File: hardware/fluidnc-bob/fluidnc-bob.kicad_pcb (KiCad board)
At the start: 2 copper layers, 45 parts, among them J1 5V-IN, J10 LIM-Z, J11 PROBE, J2 X-DRV, J3 Y-DRV, J4 Z-DRV, J5 LIM-X, J6 LIM-Y, J7 RELAY, J8 AUX, J9 SD, Q1 2N7000, U1 SN74HC541N

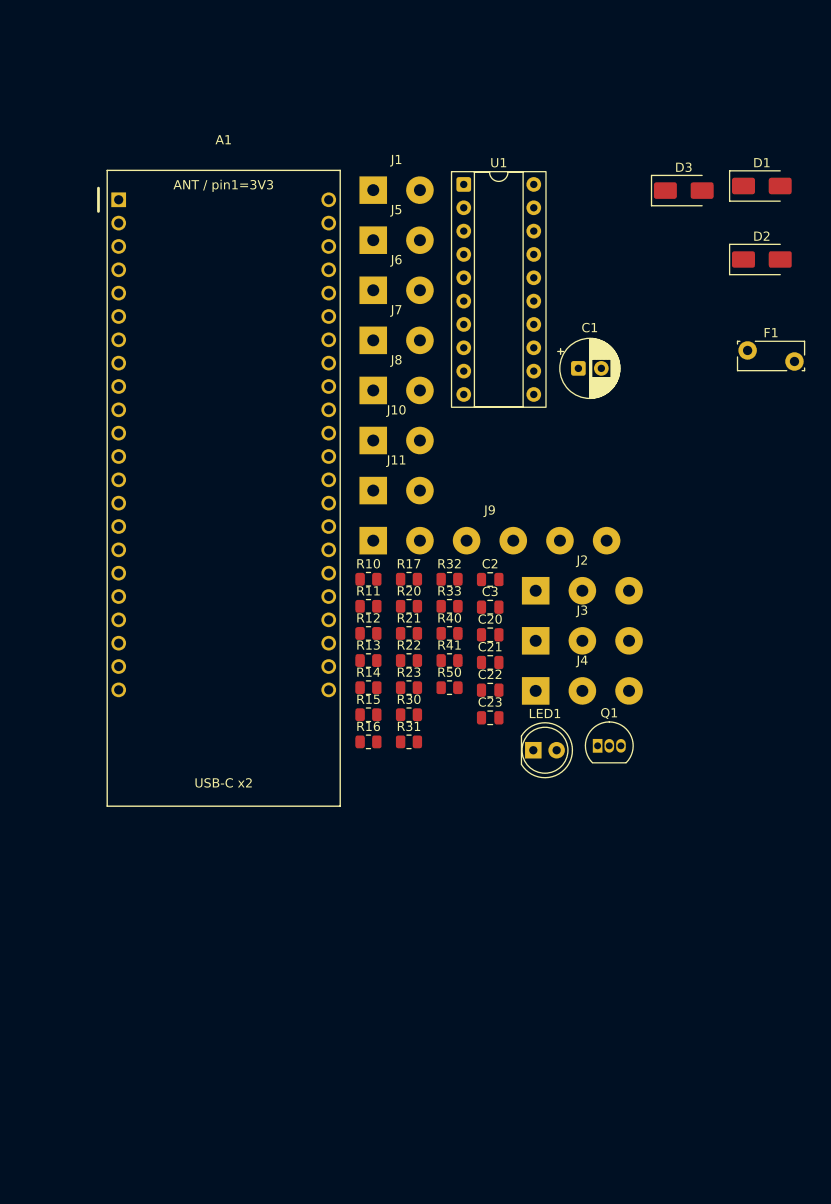
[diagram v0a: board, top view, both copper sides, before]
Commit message: Layout updated
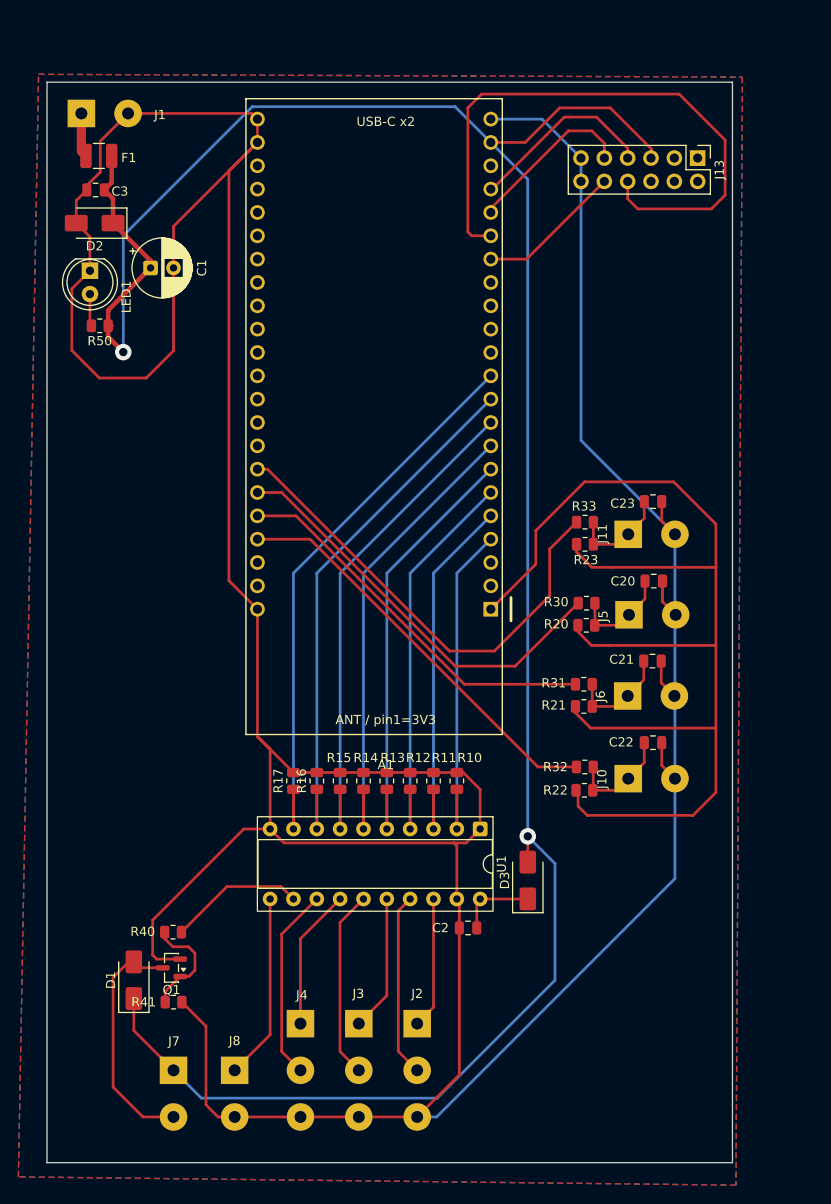
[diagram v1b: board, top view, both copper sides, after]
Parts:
- removed J9: SD, fluidnc-bob:WirePads_1x06_P5.08mm
- added J13: Conn_02x06_Odd_Even, Connector_PinHeader_2.54mm:PinHeader_2x06_P2.54mm_Vertical, F.Cu at (83.5, 21.0)
- F1: value MF-R110 1.1A -> 1210L150/16WR; footprint Fuse:Fuse_Bourns_MF-RG300 -> Fuse:Fuse_1210_3225Metric
- Q1: value 2N7000 -> MMBT2222A; footprint Package_TO_SOT_THT:TO-92_Inline -> Package_TO_SOT_SMD:SOT-23
- moved D1 110.2 mm to (22.1, 110.4), turned to 90 degrees
- moved J7 82.4 mm to (26.5, 120.2), turned to -90 degrees
- moved D3 77.0 mm to (65.0, 99.6), turned to 90 degrees
- moved J8 75.5 mm to (33.1, 120.2), turned to -90 degrees
- moved F1 73.7 mm to (18.3, 20.7)
- moved D2 72.7 mm to (17.9, 28.0), turned to 180 degrees
- moved LED1 71.1 mm to (17.4, 33.2), turned to -90 degrees
- moved U1 70.2 mm to (59.8, 94.0), turned to -90 degrees
- moved A1 68.3 mm to (61.0, 80.5), turned to 180 degrees
- moved C3 62.5 mm to (18.0, 24.4), turned to 180 degrees
- moved R50 54.8 mm to (18.4, 39.2), turned to 180 degrees
- moved Q1 52.3 mm to (26.2, 109.1), turned to 180 degrees
- moved J6 52.1 mm to (75.9, 79.5)
- moved J5 49.4 mm to (76.0, 70.7)
- moved J2 48.8 mm to (53.0, 115.2), turned to -90 degrees
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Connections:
- net Net-(U1-Y1) renamed XSTEP
- net Net-(U1-Y2) renamed XDIR
- net Net-(U1-Y4) renamed YDIR
- net Net-(U1-Y5) renamed ZSTEP
- net Net-(U1-Y7) renamed SPIN5
- net Net-(U1-Y8) renamed AUX1
- A1 pad 16: unconnected-(A1-GPIO10-Pad16) -> CS
- A1 pad 17: unconnected-(A1-GPIO11-Pad17) -> MOSI
- A1 pad 18: unconnected-(A1-GPIO12-Pad18) -> SCK
- A1 pad 19: unconnected-(A1-GPIO13-Pad19) -> MISO
- A1 pad 30: Net-(A1-GPIO40) -> unconnected-(A1-GPIO40-Pad30)
- A1 pad 31: Net-(A1-GPIO39) -> unconnected-(A1-GPIO39-Pad31)
- A1 pad 32: Net-(A1-GPIO38) -> unconnected-(A1-GPIO38-Pad32)
- A1 pad 40: Net-(A1-GPIO21) -> unconnected-(A1-GPIO21-Pad40)
- C2 pad 1: VCC_BUF -> GND
- C2 pad 2: GND -> VCC_BUF
- J3 pad 1: Net-(U1-Y6) -> YSTEP
- J4 pad 2: unconnected-(J4-Pad2) -> ZDIR
- Q1 pad 1: GND -> Net-(Q1-B)
- Q1 pad 2: Net-(Q1-G) -> GND
- R30 pad 2: Net-(A1-GPIO1) -> Net-(A1-GPIO42)
- R32 pad 2: Net-(A1-GPIO42) -> Net-(A1-GPIO1)
- R40 pad 2: Net-(Q1-G) -> Net-(Q1-B)
- R41 pad 1: Net-(Q1-G) -> Net-(Q1-B)
- U1 pad 13: Net-(U1-Y6) -> ZDIR
- U1 pad 16: unconnected-(U1-Y3-Pad16) -> YSTEP
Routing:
- net GND: track 0.00 -> 461.3 mm
- net +5V: track 0.00 -> 263.3 mm, vias 0 -> 2
- net +3V3: track 0.00 -> 131.5 mm
- net MOSI: track 0.00 -> 66.4 mm
- net Net-(A1-GPIO18): track 0.00 -> 62.5 mm
- net Net-(A1-GPIO17): track 0.00 -> 58.9 mm
- net Net-(A1-GPIO16): track 0.00 -> 55.4 mm
- net Net-(A1-GPIO15): track 0.00 -> 51.8 mm
- net Net-(A1-GPIO41): track 0.00 -> 51.7 mm
- net Net-(A1-GPIO7): track 0.00 -> 48.2 mm
- net Net-(A1-GPIO42): track 0.00 -> 45.6 mm
- net Net-(A1-GPIO1): track 0.00 -> 45.0 mm
- net Net-(A1-GPIO6): track 0.00 -> 44.6 mm
- net Net-(A1-GPIO2): track 0.00 -> 42.2 mm
- net Net-(A1-GPIO5): track 0.00 -> 41.0 mm
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- added copper zone on B.Cu, net GND
- added copper zone on F.Cu, net GND
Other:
- board outline added: 74.6 x 117.6 mm

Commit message: Layout changed to shrink
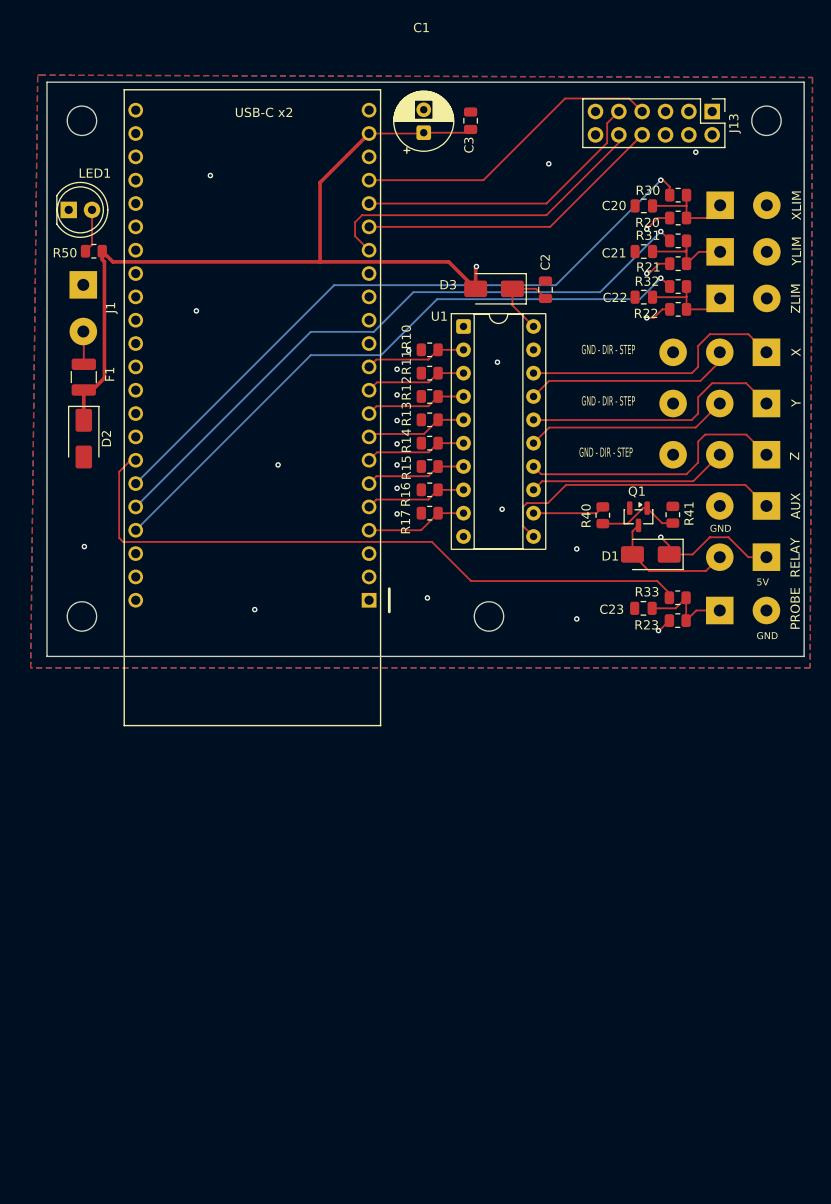
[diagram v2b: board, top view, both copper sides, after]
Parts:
- added H1: MountingHole, MountingHole:MountingHole_3.2mm_M3, F.Cu at (16.5, 16.9)
- added H2: MountingHole, MountingHole:MountingHole_3.2mm_M3, F.Cu at (91.0, 16.9)
- added H3: MountingHole, MountingHole:MountingHole_3.2mm_M3, F.Cu at (16.5, 70.8)
- added H4: MountingHole, MountingHole:MountingHole_3.2mm_M3, F.Cu at (60.8, 70.8)
- moved RELAY 85.3 mm to (91.0, 64.4), turned to 180 degrees
- moved AUX 84.4 mm to (91.0, 58.8), turned to 180 degrees
- moved X 82.4 mm to (91.0, 42.1), turned to 180 degrees
- moved Y 80.8 mm to (91.0, 47.7), turned to 180 degrees
- moved Z 80.0 mm to (91.0, 53.2), turned to 180 degrees
- moved R41 75.9 mm to (80.8, 59.8), turned to 90 degrees
- moved D1 72.9 mm to (78.4, 64.1), turned to 180 degrees
- moved Q1 70.7 mm to (77.1, 60.0), turned to -90 degrees
- moved C2 70.0 mm to (67.0, 35.3), turned to -90 degrees
- moved R40 65.2 mm to (73.2, 59.8), turned to -90 degrees
- moved D3 64.5 mm to (61.4, 35.2), turned to 180 degrees
- moved U1 54.7 mm to (58.0, 39.3), turned to 0 degrees
- moved R22 53.3 mm to (81.4, 37.4)
- moved R32 53.3 mm to (81.4, 34.9)
- moved ZLIM 53.2 mm to (86.0, 36.2)
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- renumbered J8 to AUX, J11 to PROBE, J7 to RELAY, J2 to X, J5 to XLIM, J3 to Y, J6 to YLIM, J4 to Z, J10 to ZLIM
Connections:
- J1 pad 1: Net-(F1-Pad1) -> GND
- J1 pad 2: GND -> Net-(F1-Pad1)
- R10 pad 1: Net-(A1-GPIO4) -> Net-(A1-GPIO18)
- R11 pad 1: Net-(A1-GPIO5) -> Net-(A1-GPIO17)
- R12 pad 1: Net-(A1-GPIO6) -> Net-(A1-GPIO16)
- R13 pad 1: Net-(A1-GPIO7) -> Net-(A1-GPIO15)
- R14 pad 1: Net-(A1-GPIO15) -> Net-(A1-GPIO7)
- R15 pad 1: Net-(A1-GPIO16) -> Net-(A1-GPIO6)
- R16 pad 1: Net-(A1-GPIO17) -> Net-(A1-GPIO5)
- R17 pad 1: Net-(A1-GPIO18) -> Net-(A1-GPIO4)
- U1 pad 2: Net-(A1-GPIO4) -> Net-(A1-GPIO18)
- U1 pad 3: Net-(A1-GPIO5) -> Net-(A1-GPIO17)
- U1 pad 4: Net-(A1-GPIO6) -> Net-(A1-GPIO16)
- U1 pad 5: Net-(A1-GPIO7) -> Net-(A1-GPIO15)
- U1 pad 6: Net-(A1-GPIO15) -> Net-(A1-GPIO7)
- U1 pad 7: Net-(A1-GPIO16) -> Net-(A1-GPIO6)
- U1 pad 8: Net-(A1-GPIO17) -> Net-(A1-GPIO5)
- U1 pad 9: Net-(A1-GPIO18) -> Net-(A1-GPIO4)
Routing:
- net GND: track 461.3 -> 0.58 mm, vias 0 -> 20
- net +3V3: track 131.5 -> 10.5 mm, vias 0 -> 4
- net +5V: track 263.3 -> 178.7 mm
- net Net-(A1-GPIO18): track 62.5 -> 11.0 mm
- net Net-(A1-GPIO17): track 58.9 -> 11.0 mm
- net Net-(A1-GPIO16): track 55.4 -> 11.0 mm
- net Net-(A1-GPIO15): track 51.8 -> 11.0 mm
- net Net-(A1-GPIO7): track 48.2 -> 11.0 mm
- net Net-(A1-GPIO6): track 44.6 -> 11.0 mm
- net MOSI: track 66.4 -> 33.9 mm
- net Net-(A1-GPIO5): track 41.0 -> 11.0 mm
- net Net-(A1-GPIO2): track 42.2 -> 71.0 mm, vias 0 -> 1
- net Net-(A1-GPIO42): track 45.6 -> 73.0 mm, vias 0 -> 1
- net Net-(A1-GPIO4): track 37.4 -> 11.0 mm
- net Net-(A1-GPIO1): track 45.0 -> 69.9 mm, vias 0 -> 1
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- added copper zone on In2.Cu, net +3V3
- added copper zone on In1.Cu, net GND
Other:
- board size 74.6 x 117.6 mm -> 82.4 x 62.5 mm
- copper layers 2 -> 4
- board text added: "5V"
- board text added: "GND"
- board text added: "GND - DIR - STEP"
